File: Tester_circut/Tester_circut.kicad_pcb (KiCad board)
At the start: 2 copper layers, 185.7 x 101.9 mm, 98 parts, among them J1 KF301-2P, J10 Conn_01x01_Pin, J11 KF301-2P, J12 KF301-2P, J16 Micro_SD_Card_Module, J2 KF301-2P, J3 KF301-2P, J4 KF301-2P, J5 KF301-2P, J6 KF301-2P, J7 KF301-2P, J8 KF301-2P, J9 Conn_01x01_Pin, M10 Fan, M7 Motor_Servo, M8 Motor_Servo, M9 Fan, Q2 BC547, SW1 Encoder, SW3 BtnUp, SW4 BtnDown, SW5 BtnCtr, SW6 BtnLeft, SW7 BtnRight, U1 LF90_TO220, U13 TMC2209_SILENTSTEPSTICK, U2 TMC2209_SILENTSTEPSTICK, U3 TMC2209_SILENTSTEPSTICK, U4 LCD, U5 TMC2209_SILENTSTEPSTICK, U7 LM7805_TO220, U8 LF33_TO220

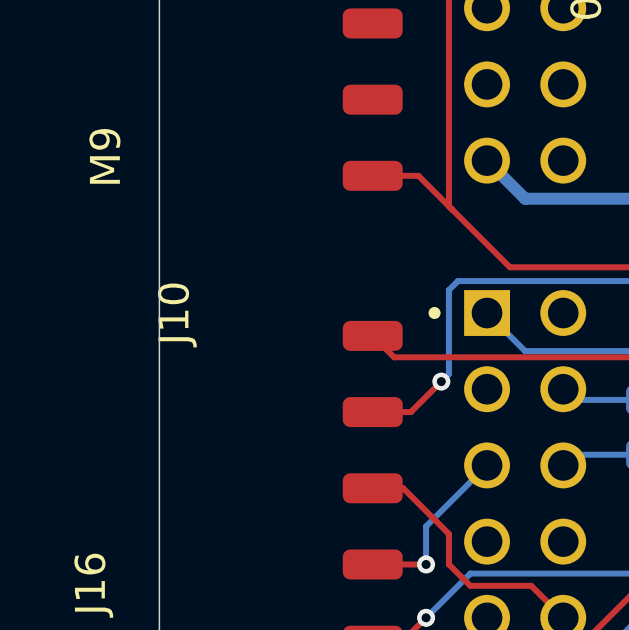
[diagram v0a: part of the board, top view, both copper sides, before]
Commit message: schematic update
probably final update
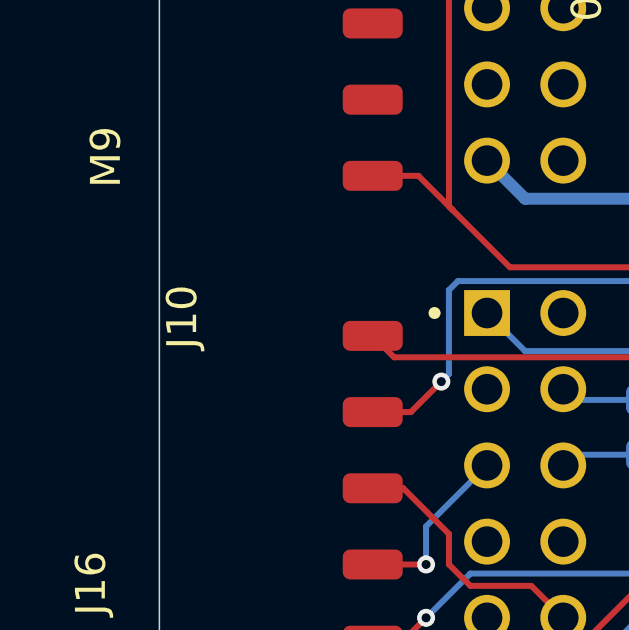
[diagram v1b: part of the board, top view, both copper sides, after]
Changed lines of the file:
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@@
 		(at 47.498 92.842 90)
 		(property "Reference" "J10"
-			(at 0.132 -0.254 90)
+			(at 0 0 90)
 			(unlocked yes)
 			(layer "F.SilkS")
@@
 		)
 		(property "Value" "Conn_01x01_Pin"
-			(at -1.646 -4.064 90)
+			(at -0.376 -4.826 90)
 			(unlocked yes)
 			(layer "F.Fab")
